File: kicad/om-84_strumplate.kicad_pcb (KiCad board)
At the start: 2 copper layers, 117.2 x 151.8 mm, 0 parts

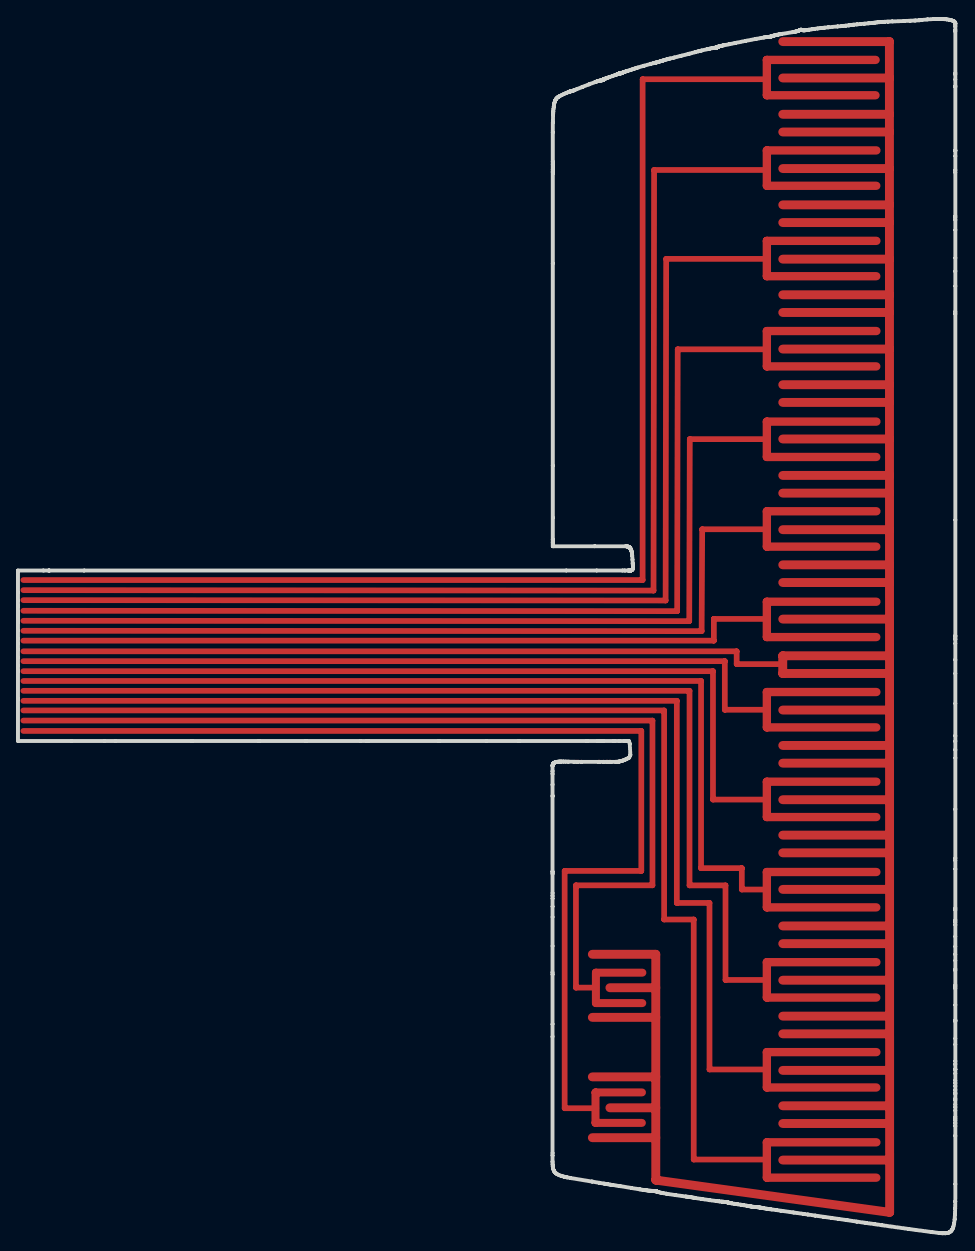
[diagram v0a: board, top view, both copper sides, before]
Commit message: Organization, Updated Gerber, officially ordered V1.0
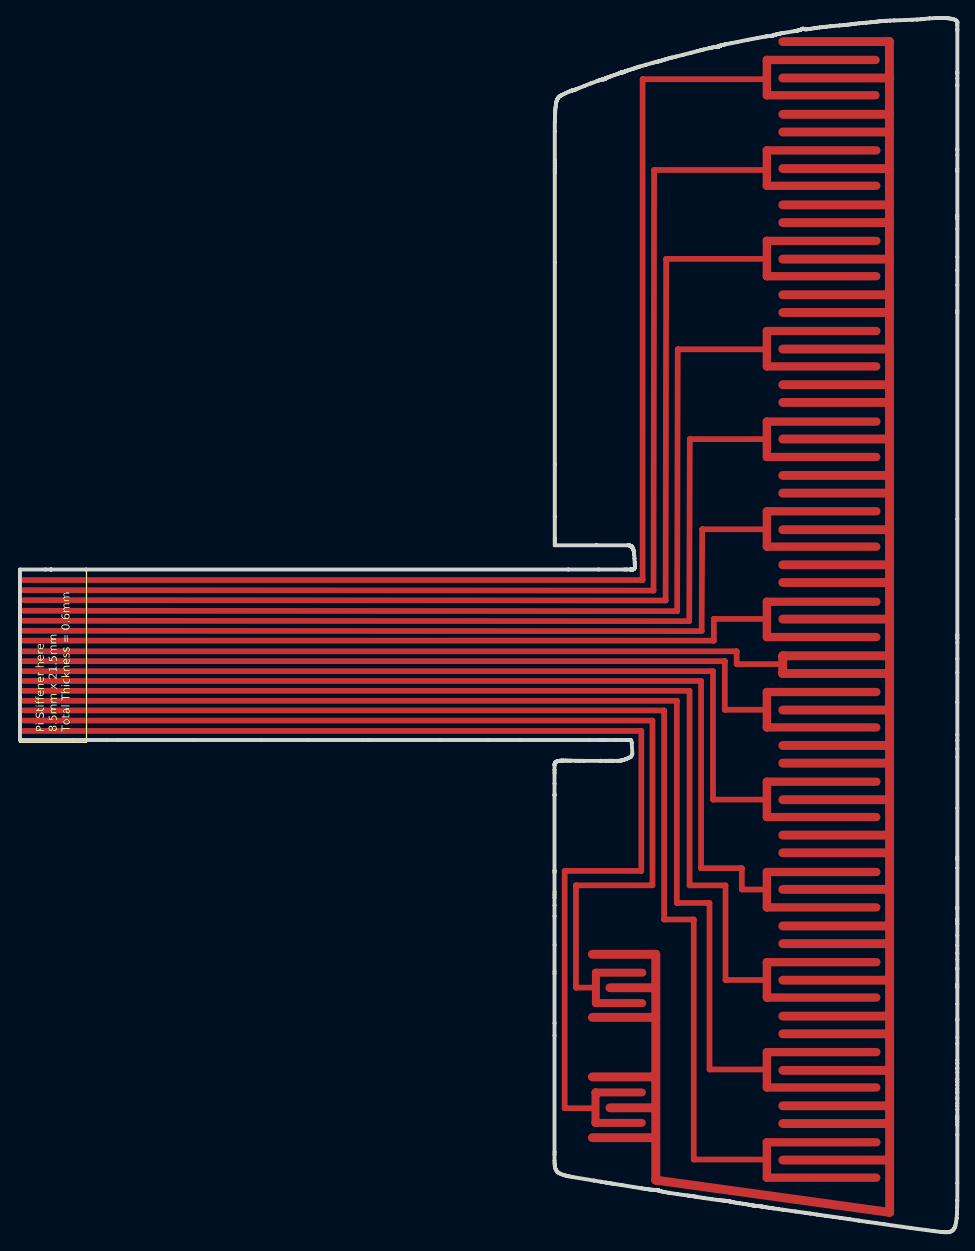
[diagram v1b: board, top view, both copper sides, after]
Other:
- board text added: "Pi Stiffener here 8.5mm x 21.5mm Total Thickness = 0.6mm"
